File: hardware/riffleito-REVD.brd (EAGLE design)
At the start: 66.8 x 18 mm, 29 parts, among them IC1 ATMEGA328P, IC2 24AA128SN, IC4 MCP1700-33, X1 16 MHz

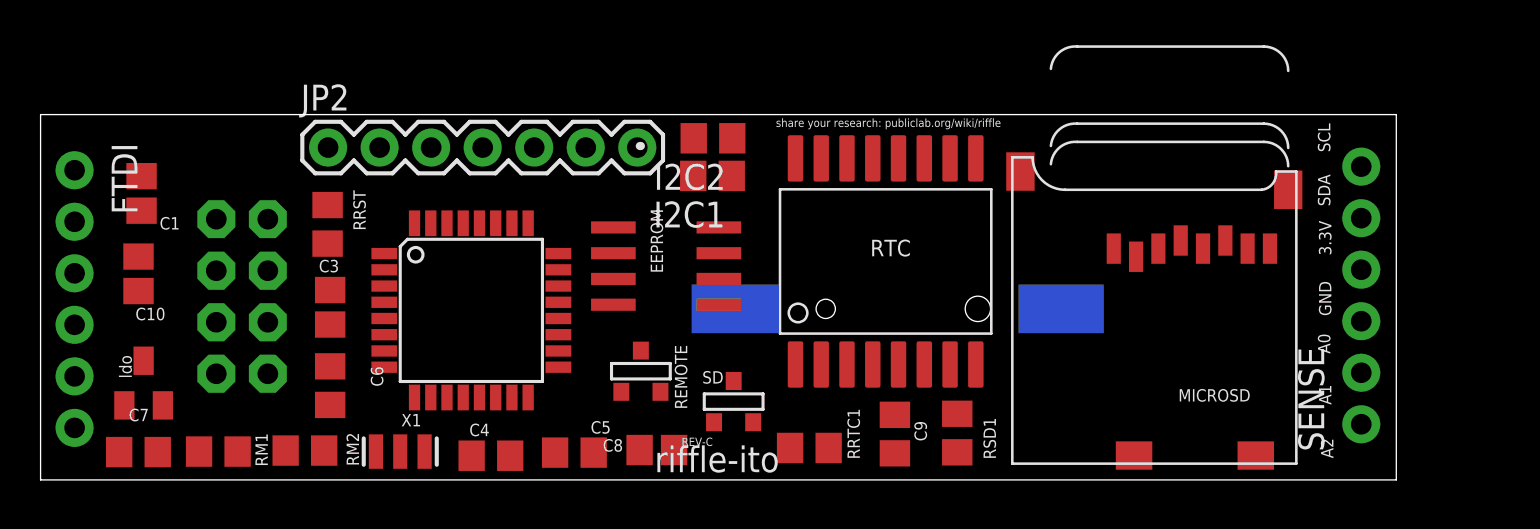
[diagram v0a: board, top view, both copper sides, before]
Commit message: routed!
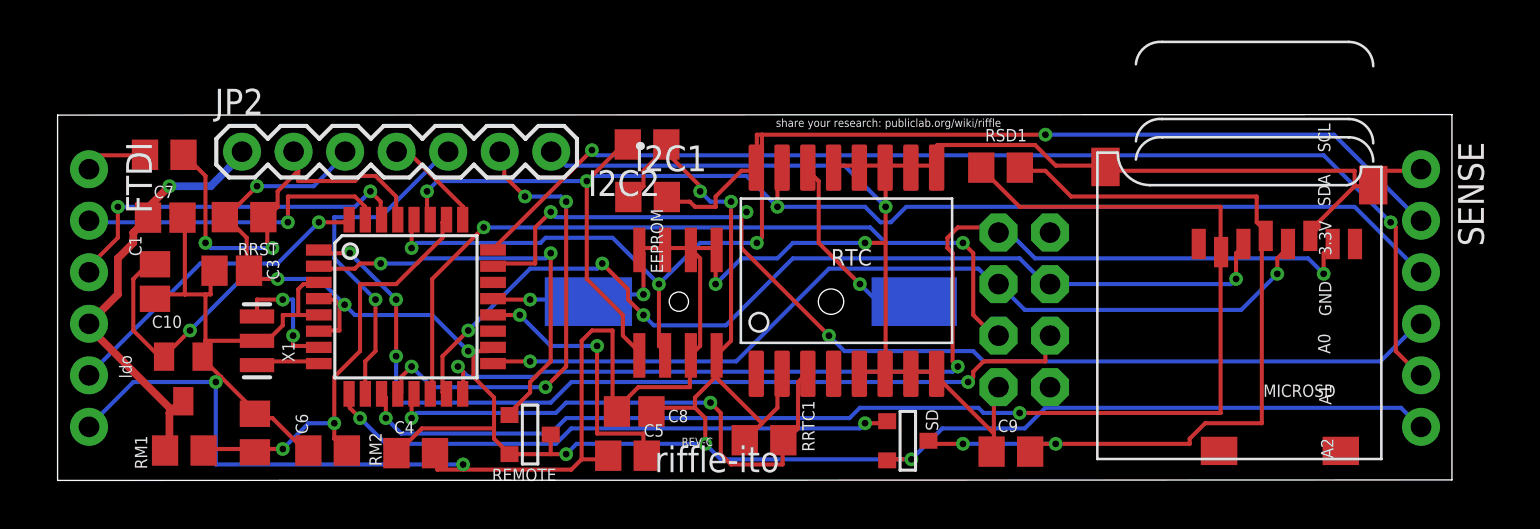
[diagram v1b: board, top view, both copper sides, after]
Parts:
- moved RAD 38.6 mm to (48.2, 8.38), turned to 90 degrees
- moved C7 14.7 mm to (5.84, 16.0), turned to 0 degrees
- moved RSD1 13.3 mm to (47.1, 15.4), turned to 0 degrees
- moved SENSE 12.9 mm to (67.8, 15.3), turned to 270 degrees
- moved X1 8.93 mm to (10.4, 6.86), turned to 270 degrees
- moved SD 8.78 mm to (42.5, 1.91), turned to 90 degrees
- moved BAT 7.25 mm to (38.7, 8.79)
- moved REMOTE 6.33 mm to (23.9, 2.21), turned to 90 degrees
- moved C9 5.78 mm to (47.6, 1.40), turned to 0 degrees
- moved C3 5.18 mm to (9.17, 10.3), turned to 180 degrees
- moved C6 4.38 mm to (10.3, 2.31)
- moved JP2 4.25 mm to (9.68, 16.2)
- moved MICROSD 4.20 mm to (65.8, 0.99)
- moved RRST 4.13 mm to (9.78, 13.0), turned to 0 degrees
- moved C4 3.71 mm to (18.2, 1.32)
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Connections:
- net A0: now also SENSE.4; no longer SENSE.5
- net A1: now also SENSE.5; no longer SENSE.6
- net GND: now also SENSE.1; no longer SENSE.4
- net SCL: now also SENSE.2; no longer SENSE.1
- net SDA: now also SENSE.3; no longer SENSE.2
- net VCC: now also SENSE.6; no longer SENSE.3
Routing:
- net GND: track 0.00 -> 184.0 mm, vias 0 -> 7
- net VCC: track 0.00 -> 134.8 mm, vias 0 -> 10
- net SCL: track 0.00 -> 71.4 mm, vias 0 -> 4
- net SDA: track 0.00 -> 67.8 mm, vias 0 -> 3
- net D7: track 0.00 -> 66.2 mm, vias 0 -> 2
- net A1: track 0.00 -> 56.0 mm, vias 0 -> 2
- net MISO: track 0.00 -> 54.6 mm, vias 0 -> 3
- net A0: track 0.00 -> 53.3 mm, vias 0 -> 3
- net MOSI: track 0.00 -> 48.4 mm, vias 0 -> 4
- net D3: track 0.00 -> 44.5 mm, vias 0 -> 4
- net SCK: track 0.00 -> 43.9 mm, vias 0 -> 2
- net VDD: track 0.00 -> 42.3 mm, vias 0 -> 2
- net D10: track 0.00 -> 38.7 mm, vias 0 -> 2
- net D5: track 0.00 -> 28.4 mm, vias 0 -> 2
- net D9: track 0.00 -> 27.4 mm, vias 0 -> 2
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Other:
- board size 66.8 x 18 mm -> 68.7 x 18 mm

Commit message: update
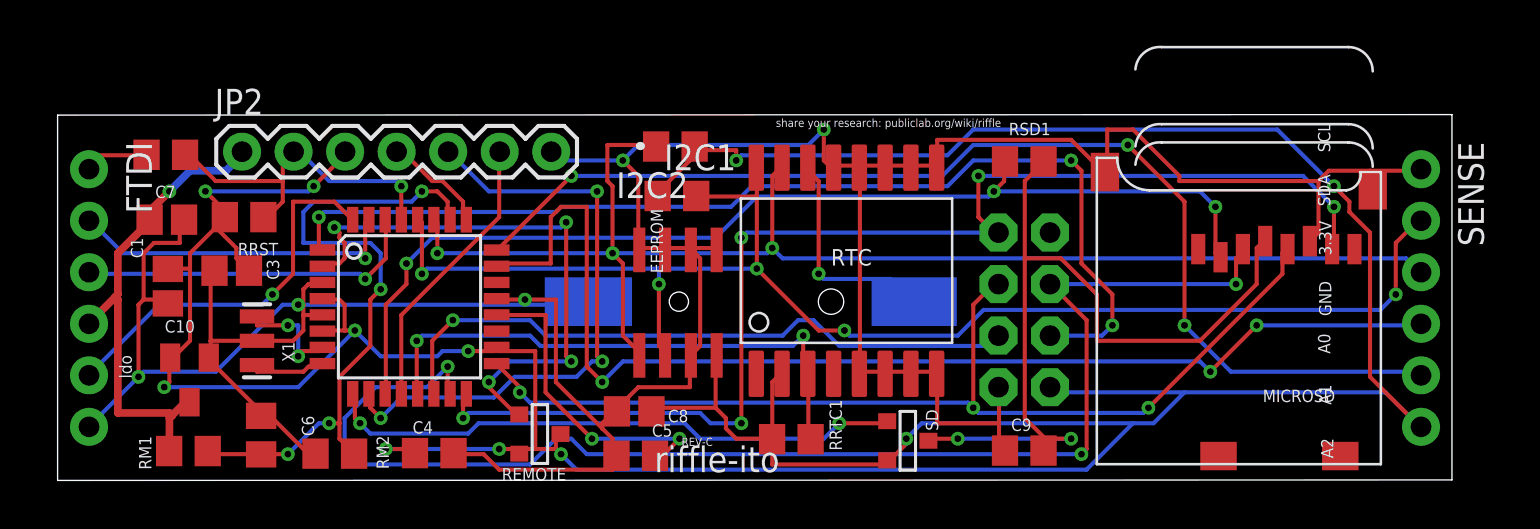
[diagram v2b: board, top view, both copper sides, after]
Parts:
- moved I2C1 1.45 mm to (31.1, 14.0)
- moved I2C2 1.40 mm to (31.0, 16.4)
- moved RRTC1 1.35 mm to (36.8, 2.01)
- moved RSD1 1.21 mm to (48.2, 15.7)
- moved C4 0.91 mm to (19.2, 1.32)
- moved C10 0.67 mm to (6.02, 9.55)
- moved C9 0.66 mm to (48.2, 1.45)
- moved REMOTE 0.48 mm to (24.4, 2.24)
- moved C5 0.41 mm to (29.1, 1.19)
- moved RM2 0.39 mm to (14.2, 1.30)
- moved C6 0.32 mm to (10.6, 2.21)
- moved IC4 0.31 mm to (7.09, 4.93)
- moved MICROSD 0.26 mm to (65.8, 0.74)
- moved RM1 0.20 mm to (7.04, 1.42)
- moved IC1 0.18 mm to (17.9, 8.53)
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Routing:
- net VCC: track 134.8 -> 200.2 mm, vias 10 -> 11
- net MOSI: track 48.4 -> 67.3 mm, vias 4 -> 3
- net D7: track 66.2 -> 52.8 mm, vias 2 -> 3
- net D6: track 16.8 -> 30.1 mm, vias 1 -> 3
- net A3: track 22.2 -> 32.4 mm, vias 2 -> 4
- net D8: track 23.1 -> 13.9 mm, vias 4 -> 0
- net D3: track 44.5 -> 52.2 mm, vias 4 -> 3
- net D4: track 20.7 -> 28.3 mm, vias 2 -> 4
- net SCK: track 43.9 -> 50.8 mm, vias 2 -> 3
- net D10: track 38.7 -> 32.4 mm, vias 2 -> 1
- net MISO: track 54.6 -> 60.8 mm, vias 3 -> 5
- net A0: track 53.3 -> 57.9 mm
- net GND: track 184.0 -> 179.6 mm, vias 7 -> 5
- net RESET: track 21.0 -> 16.9 mm, vias 2 -> 1
- net D2: track 16.0 -> 19.0 mm
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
